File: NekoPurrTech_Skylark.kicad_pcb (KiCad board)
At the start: 2 copper layers, 36.5 x 36.5 mm, 22 parts, among them IC1 ICM-42688-P, IC2 W25Q256JWPIQ, IC3 LP2992IM5-3.3, IC4 LP2992IM5-3.3, J1 Motor, J2 DJI_VTX, J3 GPS, J4 CRSF_Receiver, J5 Analog_Camera, J6 Analog_VTX, U1 STM32F405RGTx, U2 DPS310, U3 AT7456E, U4 MP9943AGQ-Z, U5 MP9943AGQ-Z

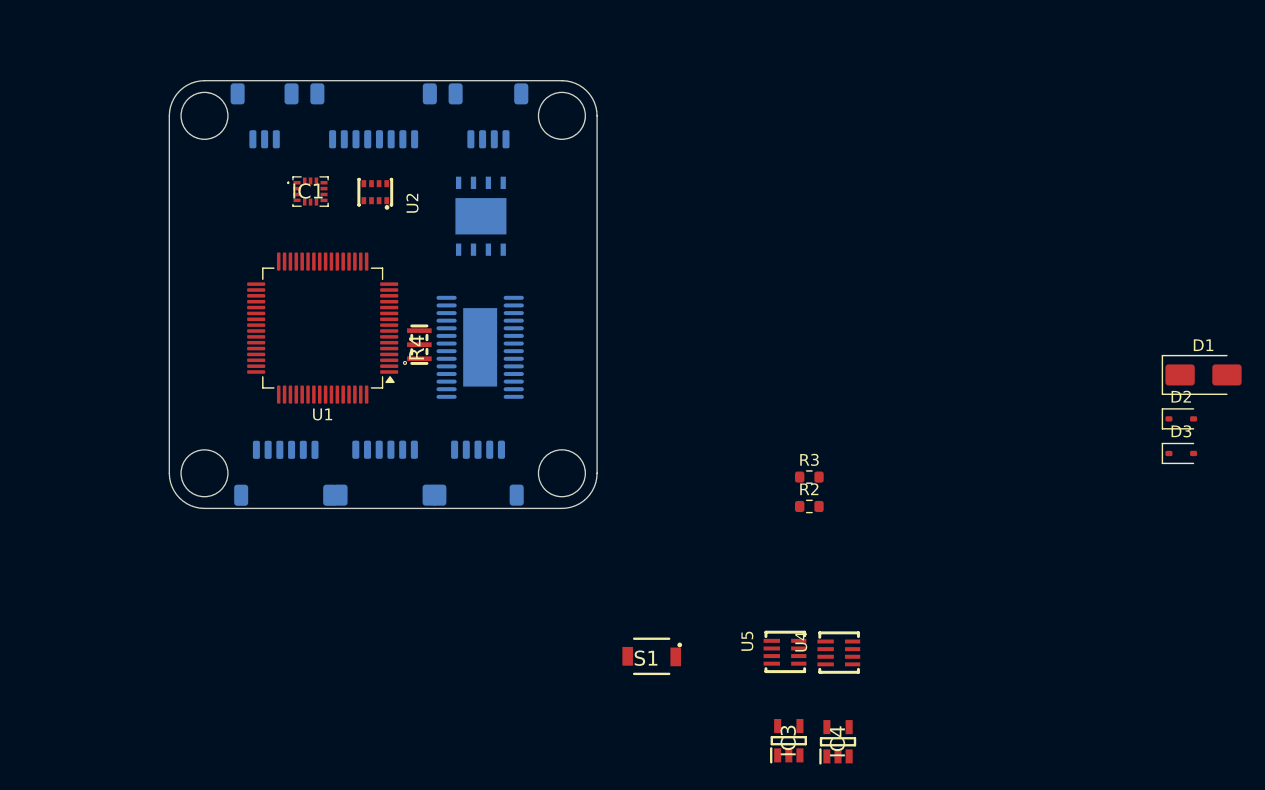
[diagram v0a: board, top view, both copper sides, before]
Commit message: Finished SCH
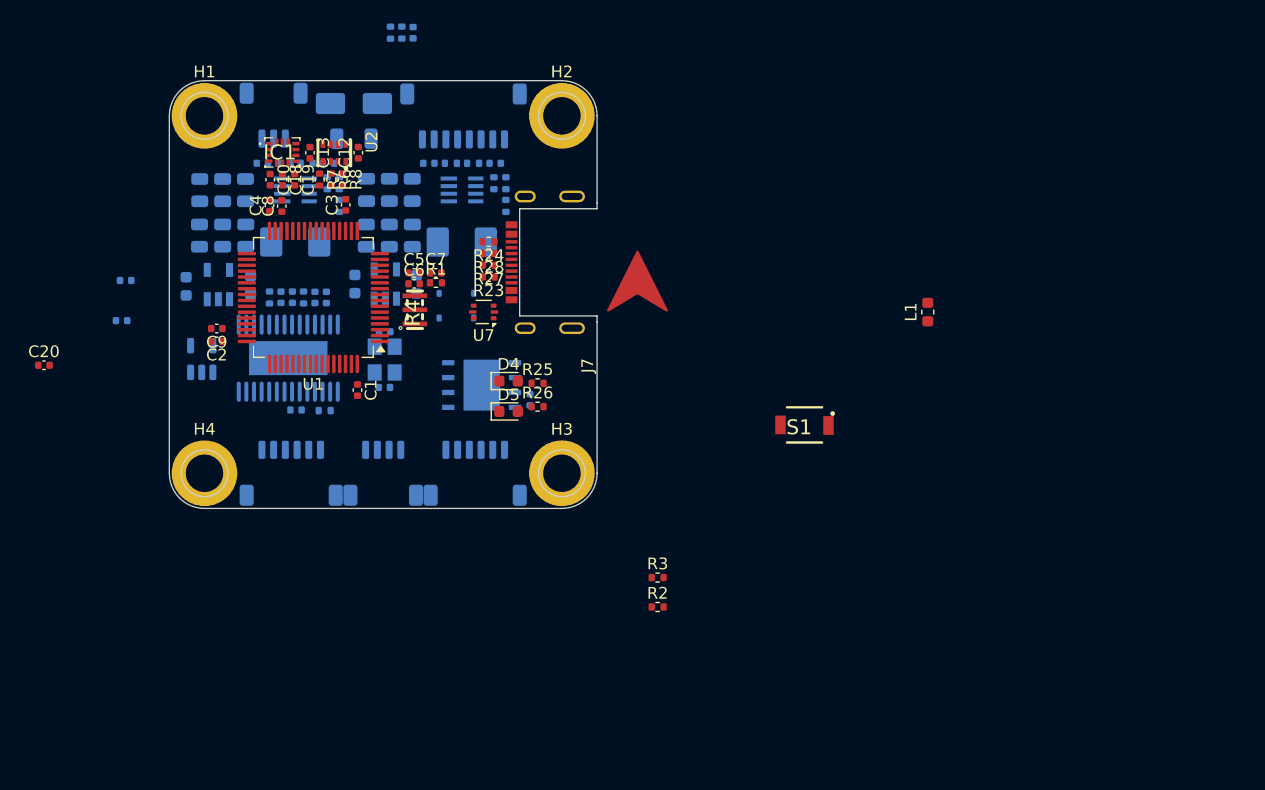
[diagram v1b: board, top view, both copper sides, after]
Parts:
- removed J6: Analog_VTX, Connector_JST:JST_SH_SM05B-SRSS-TB_1x05-1MP_P1.00mm_Horizontal
- added C1: 0.1uF, Capacitor_SMD:C_0402_1005Metric, F.Cu at (34.9, 50.8)
- added C10: 10nF, Capacitor_SMD:C_0402_1005Metric, F.Cu at (27.4, 32.8)
- added C11: 0.1uF, Capacitor_SMD:C_0402_1005Metric, B.Cu at (29.6, 52.5)
- added C12: 0.1uF, Capacitor_SMD:C_0402_1005Metric, F.Cu at (34.9, 30.5)
- added C13: 0.1uF, Capacitor_SMD:C_0402_1005Metric, F.Cu at (30.8, 30.5)
- added C14: 10uF, Capacitor_SMD:C_0402_1005Metric, B.Cu at (32.2, 42.9)
- added C15: 10uF, Capacitor_SMD:C_0402_1005Metric, B.Cu at (31.2, 42.9)
- added C16: 0.1uF, Capacitor_SMD:C_0402_1005Metric, B.Cu at (28.3, 42.9)
- added C17: 0.1uF, Capacitor_SMD:C_0402_1005Metric, B.Cu at (29.3, 42.9)
- added C18: 0.1uF, Capacitor_SMD:C_0402_1005Metric, F.Cu at (28.4, 32.8)
- added C19: 2.2uF, Capacitor_SMD:C_0402_1005Metric, F.Cu at (29.5, 32.8)
- added C2: 0.1uF, Capacitor_SMD:C_0402_1005Metric, F.Cu at (22.9, 46.6)
- added C20: 0.1uF, Capacitor_SMD:C_0402_1005Metric, F.Cu at (8.10, 48.7)
- added C21: 0.1uF, Capacitor_SMD:C_0402_1005Metric, B.Cu at (49.6, 51.6)
- added C22: 0.1uF, Capacitor_SMD:C_0402_1005Metric, B.Cu at (46.6, 31.4)
- added C23: 1uF, Capacitor_SMD:C_0603_1608Metric, B.Cu at (34.6, 41.7)
- added C24: 1uF, Capacitor_SMD:C_0603_1608Metric, B.Cu at (20.2, 41.9)
- added C25: 0.1uF, Capacitor_SMD:C_0402_1005Metric, B.Cu at (39.6, 20.3)
- added C26: 0.1uF, Capacitor_SMD:C_0402_1005Metric, B.Cu at (40.9, 31.4)
- added C27: 1uF/50V, Capacitor_SMD:C_0805_2012Metric, B.Cu at (35.6, 33.7)
- added C28: 10uF/50V, Capacitor_SMD:C_0805_2012Metric, B.Cu at (37.6, 33.7)
- added C29: 22uF, Capacitor_SMD:C_0805_2012Metric, B.Cu at (37.6, 37.6)
- added C3: 0.1uF, Capacitor_SMD:C_0402_1005Metric, F.Cu at (33.9, 35.0)
- added C30: 10nF, Capacitor_SMD:C_0402_1005Metric, B.Cu at (14.7, 44.9)
- added C31: 2.2uF, Capacitor_SMD:C_0603_1608Metric, B.Cu at (39.9, 41.8)
- added C32: 10nF, Capacitor_SMD:C_0402_1005Metric, B.Cu at (15.1, 41.4)
- added C33: 2.2uF, Capacitor_SMD:C_0603_1608Metric, B.Cu at (25.7, 41.8)
- added C34: 10uF/50V, Capacitor_SMD:C_0805_2012Metric, B.Cu at (39.5, 33.7)
- added C35: 22uF, Capacitor_SMD:C_0805_2012Metric, B.Cu at (39.5, 37.6)
- added C36: 0.1uF, Capacitor_SMD:C_0402_1005Metric, B.Cu at (32.4, 31.4)
- added C37: 0.1uF, Capacitor_SMD:C_0402_1005Metric, B.Cu at (26.7, 31.4)
- added C38: 1uF/50V, Capacitor_SMD:C_0805_2012Metric, B.Cu at (23.3, 33.7)
- added C39: 10uF/50V, Capacitor_SMD:C_0805_2012Metric, B.Cu at (25.3, 33.7)
- added C4: 0.1uF, Capacitor_SMD:C_0402_1005Metric, F.Cu at (27.4, 35.0)
- added C40: 22uF, Capacitor_SMD:C_0805_2012Metric, B.Cu at (21.4, 37.6)
- added C41: 10uF/50V, Capacitor_SMD:C_0805_2012Metric, B.Cu at (21.4, 33.7)
- added C42: 22uF, Capacitor_SMD:C_0805_2012Metric, B.Cu at (25.3, 37.6)
- added C43: 12pF, Capacitor_SMD:C_0402_1005Metric, B.Cu at (37.1, 50.6)
- added C44: 12pF, Capacitor_SMD:C_0402_1005Metric, B.Cu at (37.2, 45.8)
- added C45: 22uF, Capacitor_SMD:C_0805_2012Metric, B.Cu at (35.6, 37.6)
- added C46: 22uF, Capacitor_SMD:C_0805_2012Metric, B.Cu at (23.3, 37.6)
- added C5: 0.1uF, Capacitor_SMD:C_0402_1005Metric, F.Cu at (39.7, 40.8)
- added C6: 1uF, Capacitor_SMD:C_0402_1005Metric, F.Cu at (39.7, 41.7)
- added C7: 0.1uF, Capacitor_SMD:C_0402_1005Metric, F.Cu at (41.5, 40.8)
- added C8: 2.2uF, Capacitor_SMD:C_0402_1005Metric, F.Cu at (28.4, 35.1)
- added C9: 2.2uF, Capacitor_SMD:C_0402_1005Metric, F.Cu at (22.9, 45.5)
- added D4: LED, LED_SMD:LED_0603_1608Metric, F.Cu at (47.8, 50.0)
- added D5: LED, LED_SMD:LED_0603_1608Metric, F.Cu at (47.8, 52.6)
- added F1: 1206_3A, Resistor_SMD:R_1206_3216Metric, B.Cu at (34.5, 29.3)
- added H1: MountingHole_Pad, MountingHole:MountingHole_3.2mm_M3_DIN965_Pad, F.Cu at (21.8, 27.4)
- added H2: MountingHole_Pad, MountingHole:MountingHole_3.2mm_M3_DIN965_Pad, F.Cu at (52.3, 27.4)
- added H3: MountingHole_Pad, MountingHole:MountingHole_3.2mm_M3_DIN965_Pad, F.Cu at (52.3, 57.9)
- added H4: MountingHole_Pad, MountingHole:MountingHole_3.2mm_M3_DIN965_Pad, F.Cu at (21.8, 57.9)
- added J7: USB_C_Receptacle, SamacSys_Parts:USB-C_halfboard, F.Cu at (55.3, 45.0)
- added L1: L, Inductor_SMD:L_0603_1608Metric, F.Cu at (83.5, 44.1)
- added L2: 10uH, Inductor_SMD:L_APV_APH0530, B.Cu at (43.8, 38.2)
- added L3: 10uH, Inductor_SMD:L_APV_APH0530, B.Cu at (29.5, 38.2)
- added R1: 10K, Resistor_SMD:R_0402_1005Metric, F.Cu at (41.5, 41.6)
- added R10: 75R, Resistor_SMD:R_0402_1005Metric, B.Cu at (27.4, 42.9)
- added R11: 41.2K, Resistor_SMD:R_0402_1005Metric, B.Cu at (47.5, 35.1)
- added R12: 51K, Resistor_SMD:R_0402_1005Metric, B.Cu at (46.5, 33.1)
- added R13: 7.68K, Resistor_SMD:R_0402_1005Metric, B.Cu at (47.5, 33.1)
- added R14: 20R, Resistor_SMD:R_0402_1005Metric, B.Cu at (42.8, 31.4)
- added R15: 10K, Resistor_SMD:R_0402_1005Metric, B.Cu at (37.7, 20.3)
- added R16: 1K, Resistor_SMD:R_0402_1005Metric, B.Cu at (38.6, 20.3)
- added R17: 1M, Resistor_SMD:R_0402_1005Metric, B.Cu at (44.7, 31.4)
- added R18: 41.2K, Resistor_SMD:R_0402_1005Metric, B.Cu at (33.3, 35.1)
- added R19: 51K, Resistor_SMD:R_0402_1005Metric, B.Cu at (32.3, 33.1)
- added R20: 3.4K, Resistor_SMD:R_0402_1005Metric, B.Cu at (33.3, 33.1)
- added R21: 20R, Resistor_SMD:R_0402_1005Metric, B.Cu at (28.6, 31.4)
- added R22: 1M, Resistor_SMD:R_0402_1005Metric, B.Cu at (30.5, 31.4)
- added R23: 5K1, Resistor_SMD:R_0402_1005Metric, F.Cu at (46.0, 41.1)
- added R24: 5K1, Resistor_SMD:R_0402_1005Metric, F.Cu at (46.0, 38.1)
- added R25: 100R, Resistor_SMD:R_0402_1005Metric, F.Cu at (50.2, 50.2)
- added R26: 100R, Resistor_SMD:R_0402_1005Metric, F.Cu at (50.2, 52.2)
- added R27: 22R, Resistor_SMD:R_0402_1005Metric, F.Cu at (46.0, 40.1)
- added R28: 22R, Resistor_SMD:R_0402_1005Metric, F.Cu at (46.0, 39.1)
- added R5: 10K, Resistor_SMD:R_0402_1005Metric, B.Cu at (32.1, 52.5)
- added R6: 4K7, Resistor_SMD:R_0402_1005Metric, F.Cu at (32.6, 32.8)
- added R7: 4K7, Resistor_SMD:R_0402_1005Metric, F.Cu at (31.6, 32.8)
- added R8: 100K, Resistor_SMD:R_0402_1005Metric, F.Cu at (33.6, 32.8)
- added R9: 75R, Resistor_SMD:R_0402_1005Metric, B.Cu at (30.2, 42.9)
- added U6: 74LVC1G04, Package_TO_SOT_SMD:SOT-23-5, B.Cu at (21.6, 48.1)
- added U7: USBLC6-2P6, Package_TO_SOT_SMD:SOT-666, F.Cu at (45.6, 44.1)
- added Y1: YSX321SL, SamacSys_Parts:YSX321SL, B.Cu at (37.2, 48.2)
- D1, D2, D3, IC3, IC4: moved to B.Cu
- R2, R3: footprint Resistor_SMD:R_0603_1608Metric -> Resistor_SMD:R_0402_1005Metric
- U2: footprint Library:WLGA-8_L2.5-W2.0-P0.65-TR_DPS422 -> SamacSys_Parts:WLGA-8_L2.5-W2.0-P0.65-TR_DPS422
- U3: footprint Library:TSSOP-28_L9.7-W4.4-P0.65-LS6.4-BL-EP-2 -> SamacSys_Parts:TSSOP-28_L9.7-W4.4-P0.65-LS6.4-BL-EP-2
- U4, U5: footprint Library:QFN-8_L3.0-W3.0-P0.65 -> SamacSys_Parts:QFN-8_L3.0-W3.0-P0.65; moved to B.Cu
- moved D1 76.1 mm to (34.5, 26.3)
- moved IC4 65.7 mm to (23.0, 41.8)
- moved D2 64.1 mm to (41.8, 43.6), turned to -90 degrees
- moved D3 61.7 mm to (44.8, 43.6), turned to -90 degrees
- moved U5 57.5 mm to (29.6, 33.7), turned to -90 degrees
- moved IC3 52.0 mm to (37.2, 41.7)
- moved U4 50.9 mm to (43.8, 33.7), turned to -90 degrees
- moved J4 31.8 mm to (37.0, 57.9), turned to 180 degrees
- moved S1 23.7 mm to (73.0, 53.8)
- moved U3 16.4 mm to (28.9, 48.1), turned to 180 degrees
- moved R3 15.5 mm to (60.5, 66.8)
- moved R2 15.5 mm to (60.5, 69.3)
- moved IC2 14.4 mm to (45.5, 50.4), turned to 180 degrees
- moved J2 7.69 mm to (44.9, 57.9)
- moved J1 7.67 mm to (43.9, 27.4)
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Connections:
- J2 pad 6: SBUS -> /Connectors/SBUS_IN
- U1 pad 14: unconnected-(U1-PA0-Pad14) -> USART4_TX
- U1 pad 15: unconnected-(U1-PA1-Pad15) -> USART4_RX
- U1 pad 16: unconnected-(U1-PA2-Pad16) -> USART2_TX
- U1 pad 17: unconnected-(U1-PA3-Pad17) -> USART2_RX
- U1 pad 2: unconnected-(U1-PC13-Pad2) -> /MCU_Core/LED1
- U1 pad 25: unconnected-(U1-PC5-Pad25) -> ADC_RSSI
- U1 pad 26: unconnected-(U1-PB0-Pad26) -> MOTOR3
- U1 pad 27: unconnected-(U1-PB1-Pad27) -> MOTOR4
- U1 pad 29: unconnected-(U1-PB10-Pad29) -> MOTOR1
- U1 pad 3: unconnected-(U1-PC14-Pad3) -> /MCU_Core/LED2
- U1 pad 30: unconnected-(U1-PB11-Pad30) -> MOTOR2
- U1 pad 36: unconnected-(U1-PB15-Pad36) -> GYRO_CLK
- U1 pad 37: unconnected-(U1-PC6-Pad37) -> USART6_TX
- U1 pad 38: unconnected-(U1-PC7-Pad38) -> USART6_RX
- U1 pad 39: unconnected-(U1-PC8-Pad39) -> LED_STRIP
- U1 pad 40: unconnected-(U1-PC9-Pad40) -> I2C3_SDA
- U1 pad 41: unconnected-(U1-PA8-Pad41) -> I2C3_SCL
- U1 pad 43: unconnected-(U1-PA10-Pad43) -> USART1_RX
- U1 pad 44: unconnected-(U1-PA11-Pad44) -> USB_DN
- U1 pad 45: unconnected-(U1-PA12-Pad45) -> USB_DP
- U1 pad 46: unconnected-(U1-PA13-Pad46) -> SWDIO
- U1 pad 49: unconnected-(U1-PA14-Pad49) -> SWCLK
- U1 pad 51: unconnected-(U1-PC10-Pad51) -> USART3_TX
- U1 pad 52: unconnected-(U1-PC11-Pad52) -> USART3_RX
- U1 pad 54: unconnected-(U1-PD2-Pad54) -> USART5_RX
- U1 pad 61: unconnected-(U1-PB8-Pad61) -> CAMERA_CTRL
- U1 pad 62: unconnected-(U1-PB9-Pad62) -> BEEPER
- U1 pad 8: unconnected-(U1-PC0-Pad8) -> ADC_VBAT
- U1 pad 9: unconnected-(U1-PC1-Pad9) -> ADC_CURR
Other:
- outline, holes or cut-outs redrawn

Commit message: Updated PCB Layout
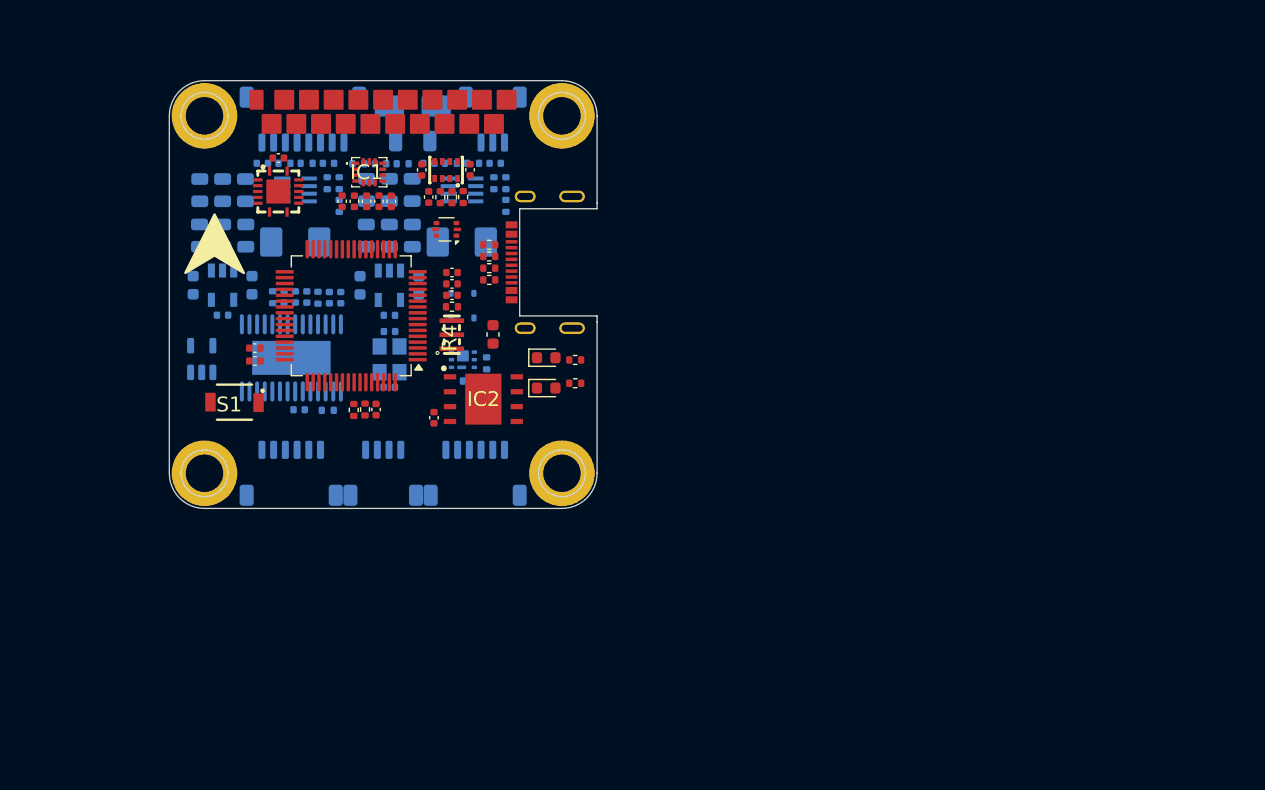
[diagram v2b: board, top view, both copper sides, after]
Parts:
- added C47: 0.1uF, Capacitor_SMD:C_0402_1005Metric, F.Cu at (28.1, 31.0)
- added Q1: CSD17313Q2, Package_SON:Texas_DQK, B.Cu at (43.9, 48.2)
- added R29: 22R, Resistor_SMD:R_0402_1005Metric, B.Cu at (45.9, 48.5)
- added R30: 10K, Resistor_SMD:R_0402_1005Metric, B.Cu at (44.4, 50.0)
- added U8: SN74LV4T125RGYR, Library:VQFN-14_L3.5-W3.5-P0.50-BL-EP, F.Cu at (28.1, 33.8)
- C20: moved to B.Cu
- C21, IC2: moved to F.Cu
- moved S1 48.7 mm to (24.4, 51.8)
- moved L1 37.1 mm to (46.4, 46.0)
- moved R2 30.9 mm to (34.5, 52.5), turned to -90 degrees
- moved R3 28.8 mm to (35.5, 52.5), turned to -90 degrees
- moved C20 23.2 mm to (30.5, 42.9), turned to 90 degrees
- moved C30 22.9 mm to (37.6, 44.4)
- moved J5 18.7 mm to (46.4, 27.7)
- moved J1 13.7 mm to (30.2, 27.7)
- moved R16 11.8 mm to (34.9, 31.5), turned to 180 degrees
- moved C25 11.5 mm to (36.8, 31.5), turned to 0 degrees
- moved R15 11.2 mm to (38.7, 31.5), turned to 180 degrees
- moved R6 10.4 mm to (42.9, 34.3)
- moved R8 10.4 mm to (43.9, 34.3)
- moved R7 10.4 mm to (41.9, 34.3)
- moved C12 9.65 mm to (44.5, 32.0)
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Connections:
- J1 pad 4: UART5_RX -> USART5_RX
- J1 pad 5: MOTOR_1 -> MOTOR1_OUT
- J1 pad 6: MOTOR_2 -> MOTOR2_OUT
- J1 pad 7: MOTOR_3 -> MOTOR3_OUT
- J1 pad 8: MOTOR_4 -> MOTOR4_OUT
- J2 pad 1: VCC_10V -> VTX_VCC
- U1 pad 4: unconnected-(U1-PC15-Pad4) -> VTX_PW_SW
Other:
- board text added: "${REFERENCE}"

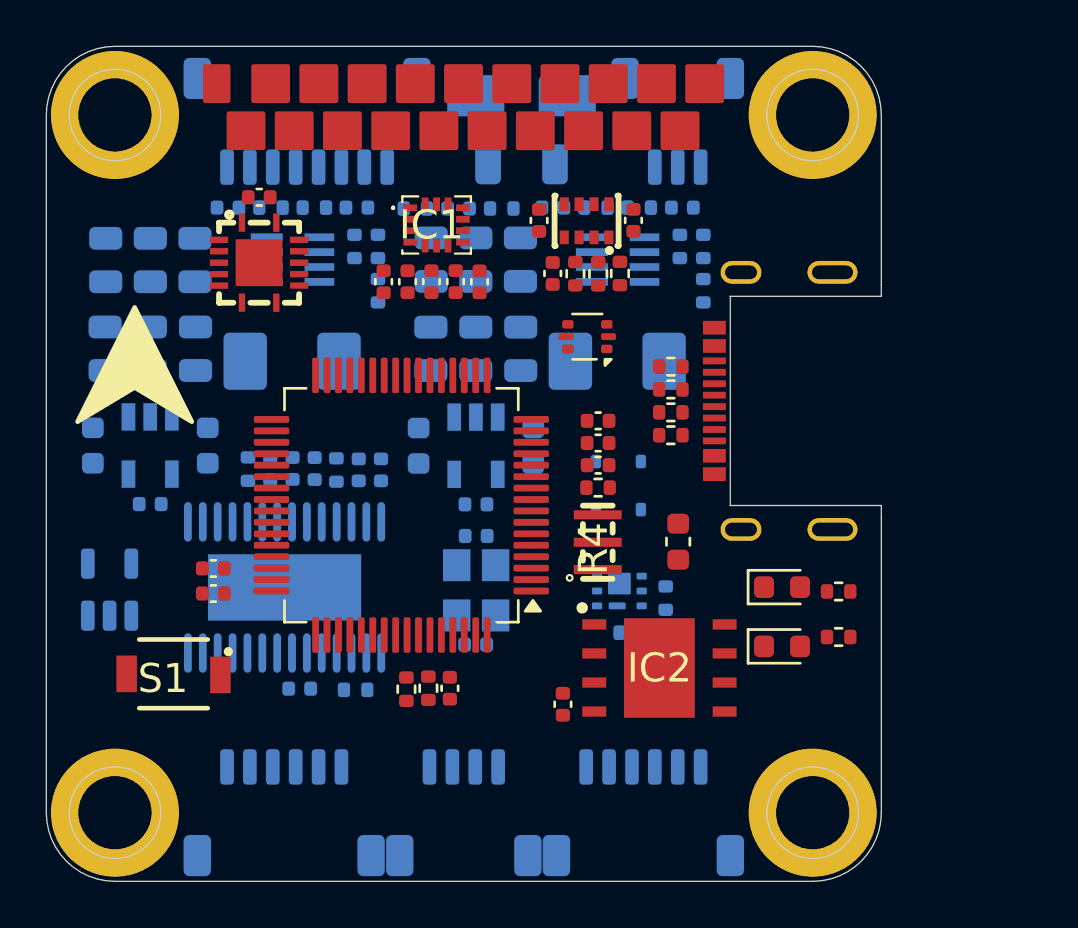
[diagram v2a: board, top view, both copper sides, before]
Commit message: Update PCB Layout
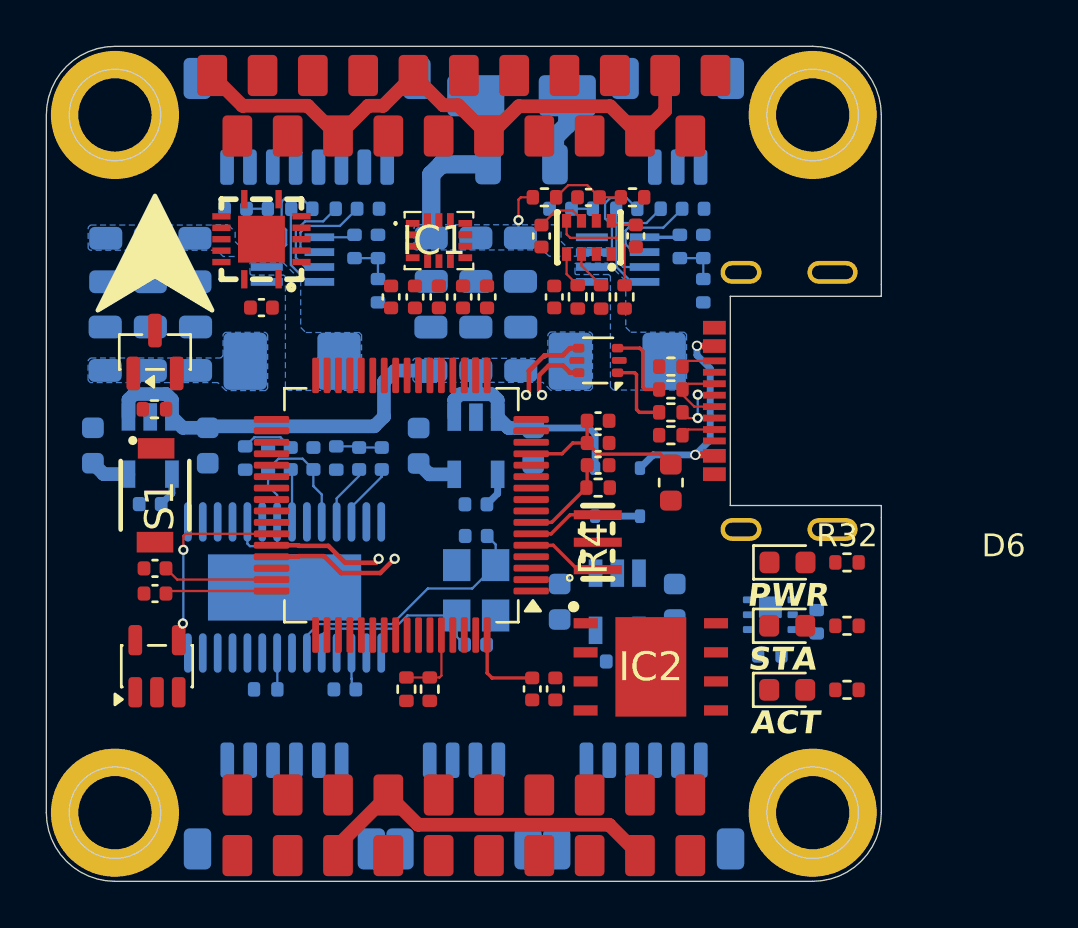
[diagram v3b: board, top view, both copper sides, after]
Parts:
- added C48: 1uF, Capacitor_SMD:C_0603_1608Metric, B.Cu at (46.3, 48.7)
- added C49: 10nF, Capacitor_SMD:C_0402_1005Metric, B.Cu at (43.8, 51.3)
- added C50: 2.2uF, Capacitor_SMD:C_0603_1608Metric, B.Cu at (41.2, 48.7)
- added D6: LED, LED_SMD:LED_0603_1608Metric, F.Cu at (51.2, 47.0)
- added IC5: LP2992IM5-3.3, Library:SOT95P280X145-5N, B.Cu at (43.8, 48.7)
- added J6: Conn_01x21_Pin, Library:Betaflight_Pad_F, F.Cu at (37.0, 27.0)
- added J8: Conn_01x20_Pin, Library:Betaflight_Pad_B, F.Cu at (37.1, 58.5)
- added Q2: SS8050, Package_TO_SOT_SMD:SOT-23, F.Cu at (23.6, 37.8)
- added R31: 1K, Resistor_SMD:R_0402_1005Metric, F.Cu at (23.5, 40.3)
- added R32: 100R, Resistor_SMD:R_0402_1005Metric, F.Cu at (53.8, 47.0)
- C25, R15, R16, U6: moved to F.Cu
- moved R16 9.51 mm to (44.4, 31.0), turned to 0 degrees
- moved S1 7.85 mm to (23.6, 44.0), turned to 90 degrees
- moved R29 6.68 mm to (52.5, 49.5)
- moved Q1 6.68 mm to (50.5, 49.2)
- moved R30 6.14 mm to (50.4, 51.0)
- moved C25 5.70 mm to (42.5, 31.0), turned to 180 degrees
- moved C47 4.83 mm to (28.2, 35.8), turned to 0 degrees
- moved U6 3.94 mm to (23.6, 51.5)
- moved R5 3.93 mm to (28.4, 52.5)
- moved C1 3.60 mm to (40.0, 52.5)
- moved L1 2.60 mm to (46.1, 43.5)
- moved C2 2.55 mm to (23.6, 48.3)
- moved C9 2.55 mm to (23.6, 47.2)
- moved R26 2.34 mm to (53.8, 52.5)
- moved D3 2.02 mm to (42.8, 43.9), turned to 90 degrees
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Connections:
- C11 pad 1: +5V -> VCC_IN
- C17 pad 1: +5V -> VCC_IN
- C20 pad 1: +5V -> VCC_IN
- C23 pad 1: VCC_5V_IN -> VCC_5V
- C24 pad 1: VCC_5V_IN -> VCC_5V
- IC3 pad 1: VCC_5V_IN -> VCC_5V
- IC3 pad 3: VCC_5V_IN -> VCC_5V
- IC4 pad 1: VCC_5V_IN -> VCC_5V
- IC4 pad 3: VCC_5V_IN -> VCC_5V
- J3 pad 5: I2C3_SDA -> I2C1_SDA
- J3 pad 6: I2C3_SCL -> I2C1_SCL
- R25 pad 2: +3.3V -> +3.3V_MCU
- R26 pad 2: +3.3V -> +3.3V_MCU
- R6 pad 1: BARO_SDA -> I2C1_SDA
- R7 pad 1: BARO_SCL -> I2C1_SCL
- S1 pad 2: +3.3V -> +3.3V_MCU
- U1 pad 39: LED_STRIP -> SERVO1
- U1 pad 40: I2C3_SDA -> SERVO2
- U1 pad 41: I2C3_SCL -> unconnected-(U1-PA8-Pad41)
- U1 pad 58: BARO_SCL -> I2C1_SCL
- U1 pad 59: BARO_SDA -> I2C1_SDA
- U2 pad 3: BARO_SDA -> I2C1_SDA
- U2 pad 4: BARO_SCL -> I2C1_SCL
- U3 pad 19: +5V -> VCC_IN
- U3 pad 21: +5V -> VCC_IN
- U3 pad 24: +5V -> VCC_IN
- U3 pad 3: +5V -> VCC_IN
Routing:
- net VCC_IN: track 0.00 -> 56.0 mm
- net VCC_5V: track 0.00 -> 27.8 mm
- net USB_DP: track 0.00 -> 23.5 mm, vias 0 -> 2
- net USB_DN: track 0.00 -> 23.4 mm, vias 0 -> 2
- net VBAT_IN: track 0.00 -> 17.2 mm, vias 0 -> 1
- net /Sensors/OSC_OUT: track 0.00 -> 11.7 mm
- net +3.3V_MCU: track 0.00 -> 10.1 mm
- net VCC_5V_USB: track 0.00 -> 9.56 mm, vias 0 -> 2
- net /Power/EN: track 0.00 -> 9.34 mm
- net USART1_RX: track 0.00 -> 8.54 mm, vias 0 -> 2
- net /Sensors/OSC_IN: track 0.00 -> 8.46 mm
- net +3.3VA_MCU: track 0.00 -> 7.66 mm
- net +3.3V_SENSOR: track 0.00 -> 5.24 mm
- net Net-(U2-SDO): track 0.00 -> 5.05 mm
- net /MCU_Core/VCAP_2: track 0.00 -> 4.82 mm
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- added copper zone on B.Cu, net Net-(U4-SW)
- added copper zone on B.Cu, net Net-(U5-SW)
- added copper zone on B.Cu, net VBAT_IN
- added copper zone on B.Cu, net VCC_10V
- added copper zone on B.Cu, net VCC_5V
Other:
- copper layers 2 -> 4
- board text added: "ACT"
- board text added: "PWR"
- board text added: "STA"
